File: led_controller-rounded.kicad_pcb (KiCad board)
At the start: 2 copper layers, 88.9 x 46.2 mm, 83 parts, among them J1 Screw_Terminal_01x02, J10 Conn_01x03, J2 SJ-3524-SMT, J3 Conn_01x03, J4 Conn_01x03, J5 Conn_01x03, J6 Conn_01x03, J7 Conn_01x03, J8 Conn_01x03, J9 Conn_01x03, SW1 RotaryEncoder_Switch, U1 MAX9814, U2 74HCT245, U3 Teensy4.0, U4 Adafruit_TFT_1in3_ST7789

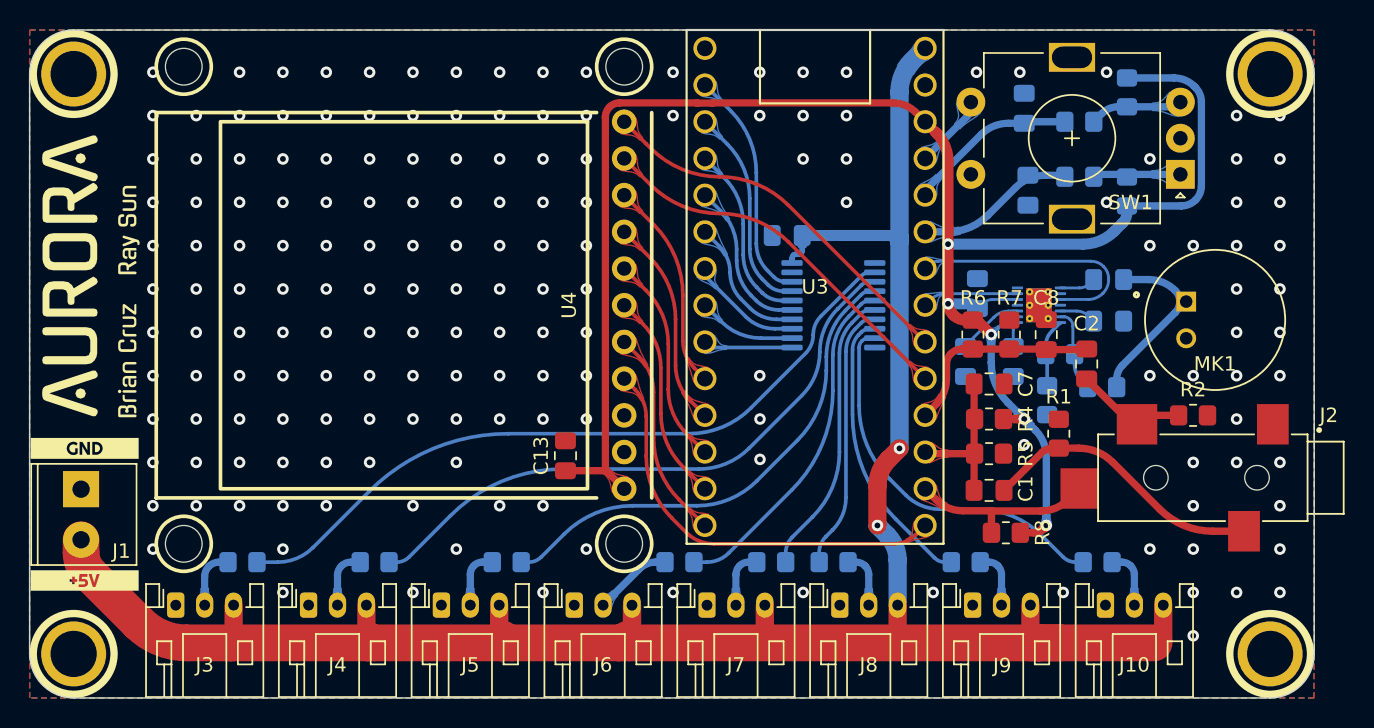
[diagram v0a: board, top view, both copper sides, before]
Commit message: verified by Brian, create gerbers
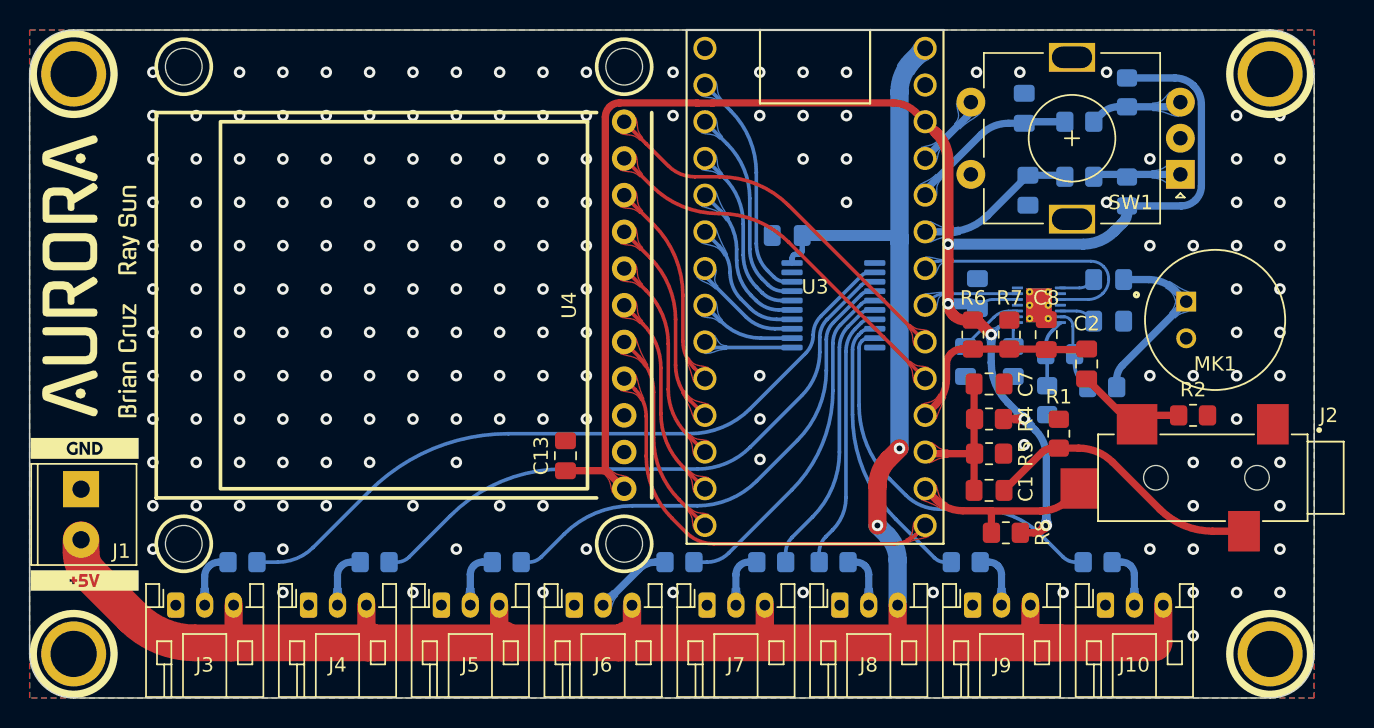
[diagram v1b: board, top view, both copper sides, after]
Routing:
- net Net-(C3-Pad2): track 12.2 -> 12.7 mm
